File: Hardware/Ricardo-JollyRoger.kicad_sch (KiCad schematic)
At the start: 47 parts, among them J1 RBUS, J3 Conn_01x08_Pin, J4 Conn_01x02_Pin, U1 ESP32-S3, U7 LM66200DRLR, Y1 R940000171

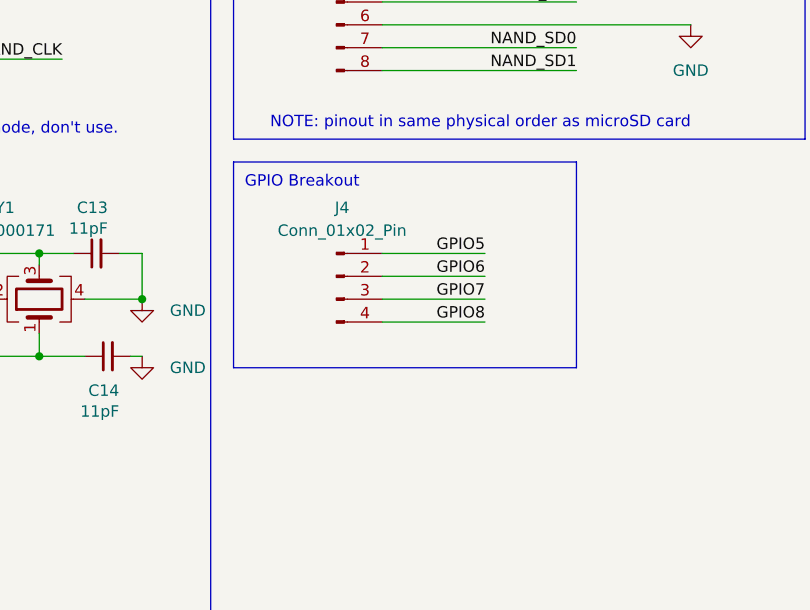
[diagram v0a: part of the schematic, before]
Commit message: Added 3V3 and GND to GPIO breakout
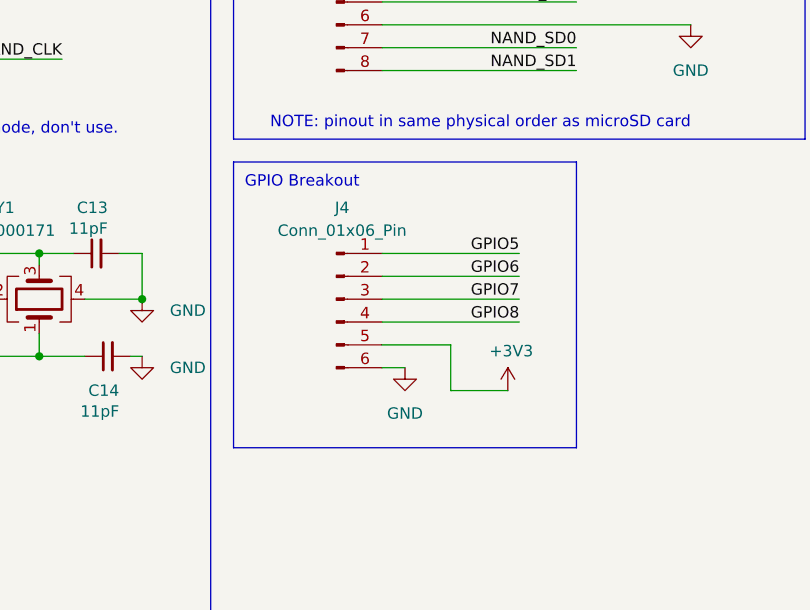
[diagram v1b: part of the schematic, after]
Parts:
- J4: value Conn_01x02_Pin -> Conn_01x06_Pin; footprint Connector_Molex:Molex_Pico-Clasp_202396-0407_1x04-1MP_P1.00mm_Horizontal -> Connector_Molex:Molex_Pico-Clasp_202396-0607_1x06-1MP_P1.00mm_Horizontal; symbol Connector:Conn_01x04_Pin -> Connector:Conn_01x06_Pin
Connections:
- net +3V3: now also J4.5 (Pin_5)
- net GND: now also J4.6 (Pin_6)
